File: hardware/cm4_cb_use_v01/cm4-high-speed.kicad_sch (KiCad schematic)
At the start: 5 parts, among them J4 USB_OTG, U2 TPD2EUSB30

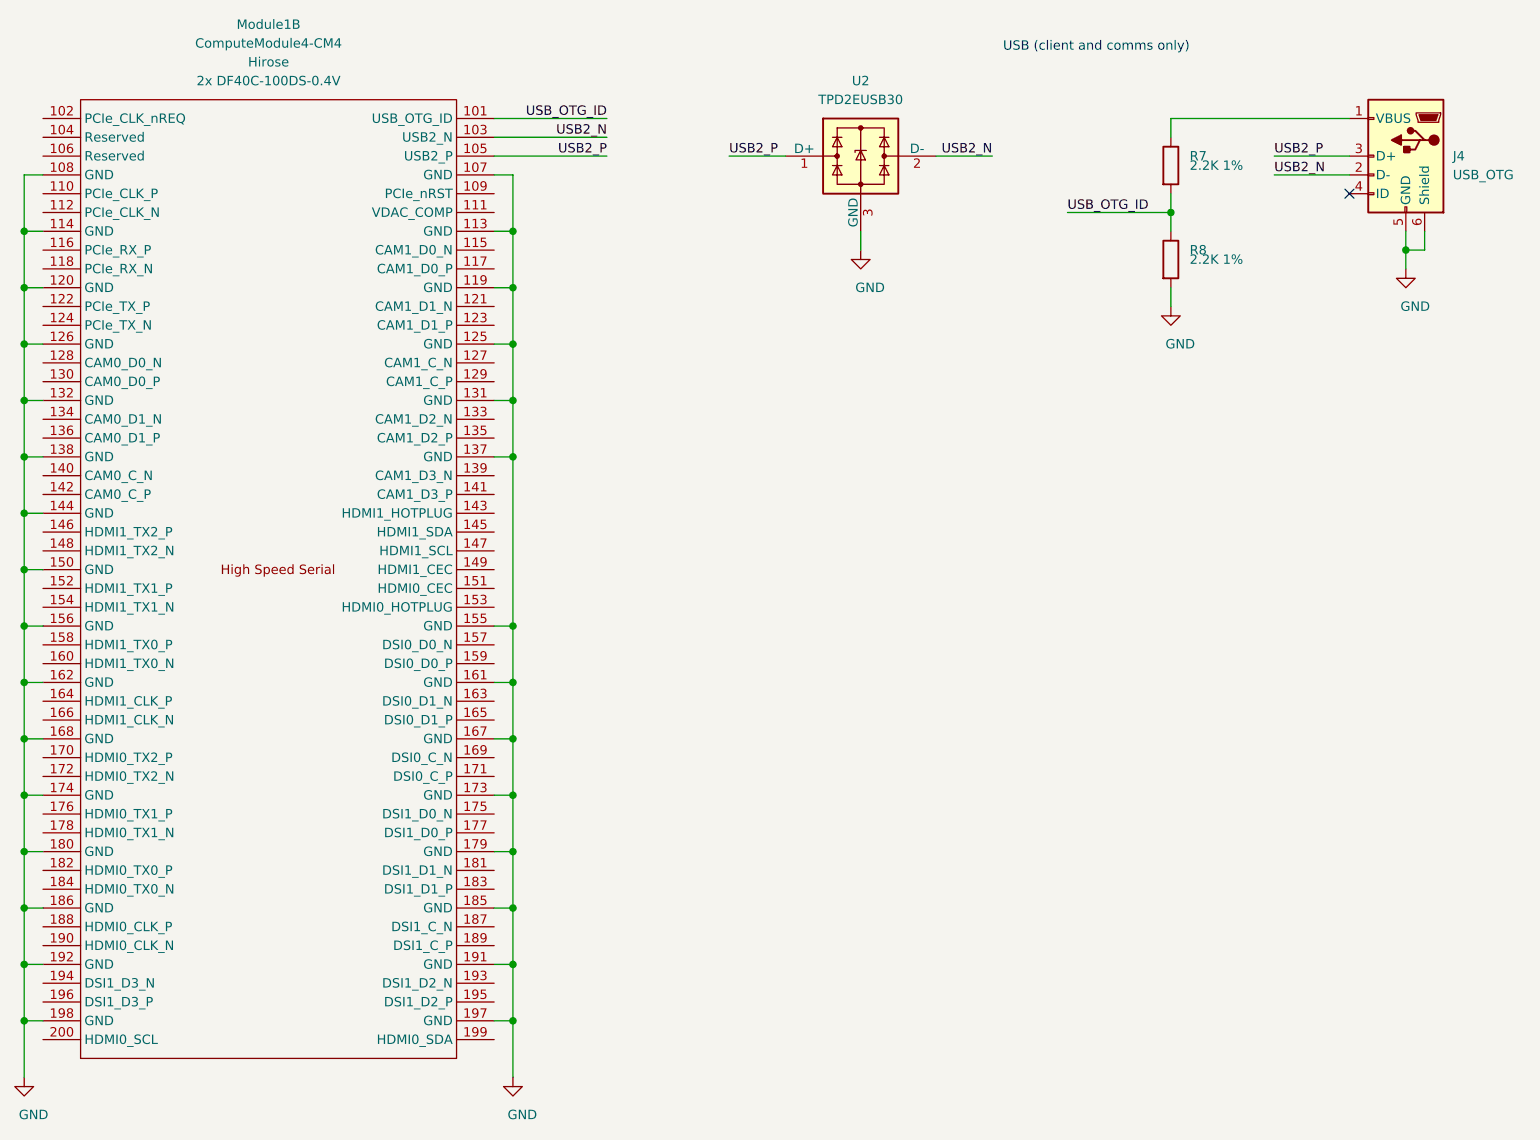
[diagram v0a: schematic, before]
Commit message: New repo
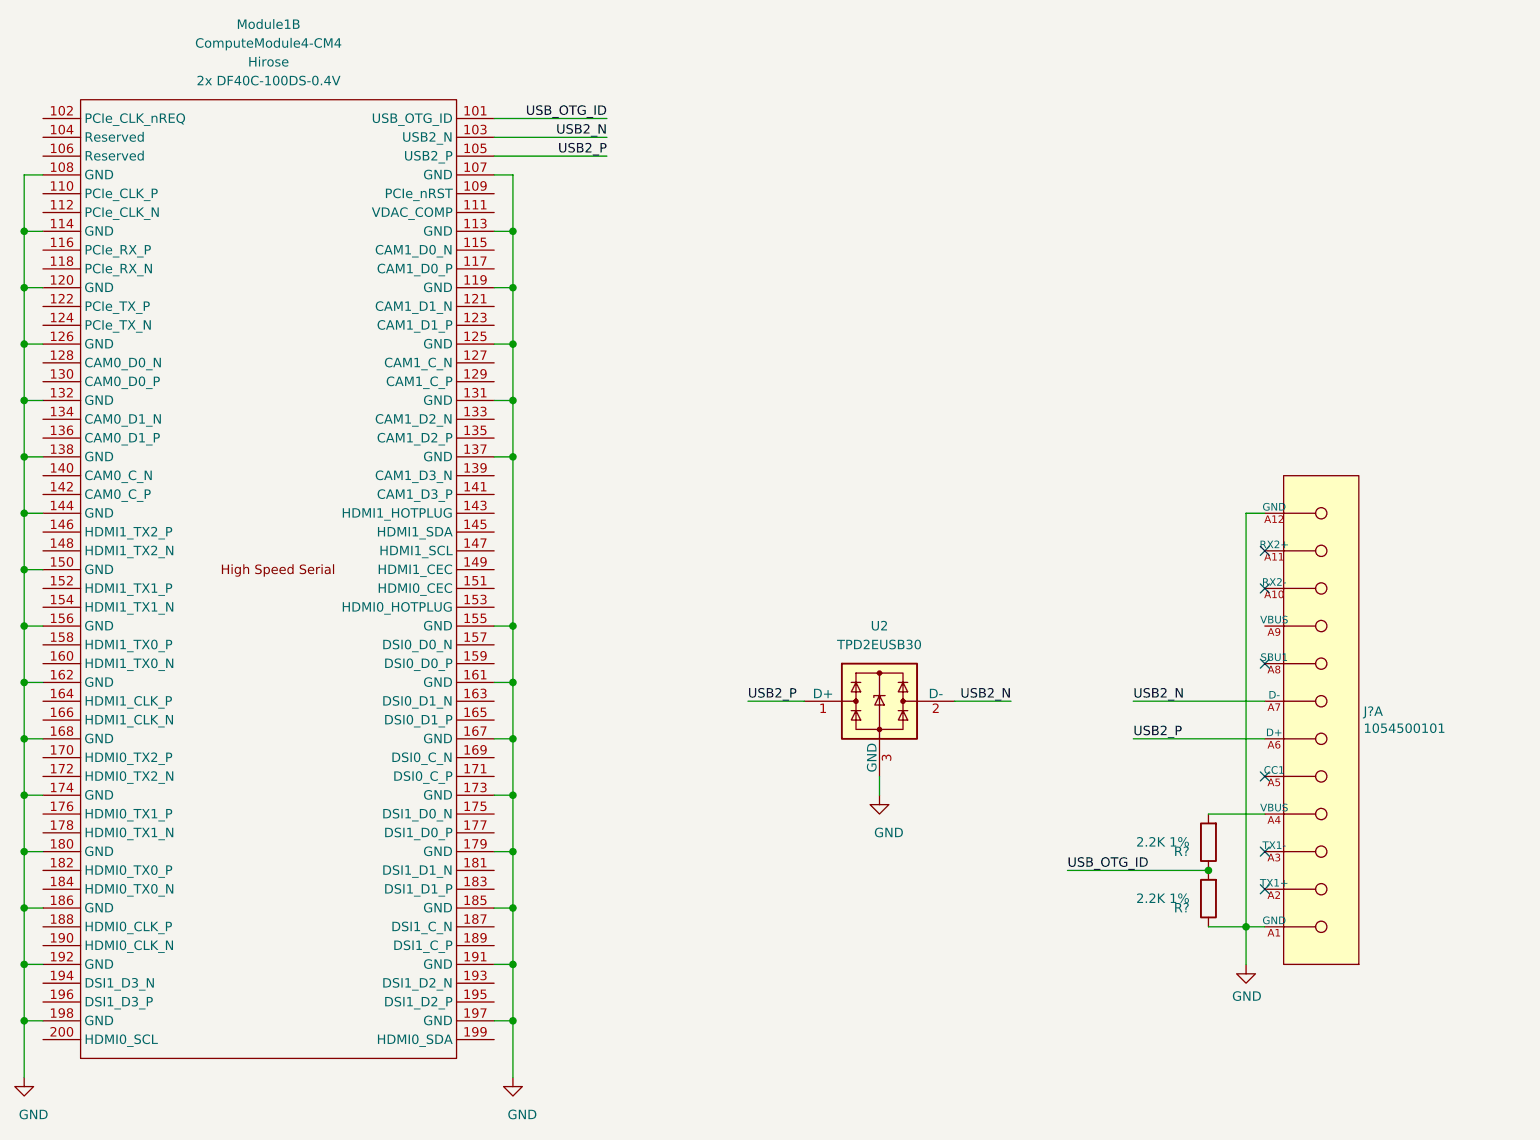
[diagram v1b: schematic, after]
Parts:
- removed J4: USB_OTG, CM4IO:USB_Micro-B_EDAC_UCON00686, symbol Connector:USB_OTG
- removed R7, R8: 2.2K 1%, Resistor_SMD:R_0603_1608Metric_Pad0.98x0.95mm_HandSolder, symbol Device:R
- added J?: 1054500101, Molex-1054500101-*, symbol MOLEX_1054500101_usb_c:1054500101
- added R? (x2): 2.2K 1%, Resistor_SMD:R_0603_1608Metric_Pad0.98x0.95mm_HandSolder, symbol Device:R
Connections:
- net GND: now also J?.A1 (GND), J?.A12 (GND), R?.1
- net USB2_N: now also J?.A7 (D-)
- net USB2_P: now also J?.A6 (D+)
- net USB_OTG_ID: now also R?.1, R?.2
- new net: J?.A4 (VBUS), R?.2
- no-connect marks 1 -> 6
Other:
- note removed: "USB (client and comms only)"
- title: Raspberry Pi Compute Module 4 Base Carrier -> Compute Module 4 Carrierboard Utskytningsenhet
- moved on the sheet: U2
